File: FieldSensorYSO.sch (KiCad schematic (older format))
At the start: 3 parts, among them J1 22-28-4023, J2 22-28-4023, Y1 Field_Sensor_54_22

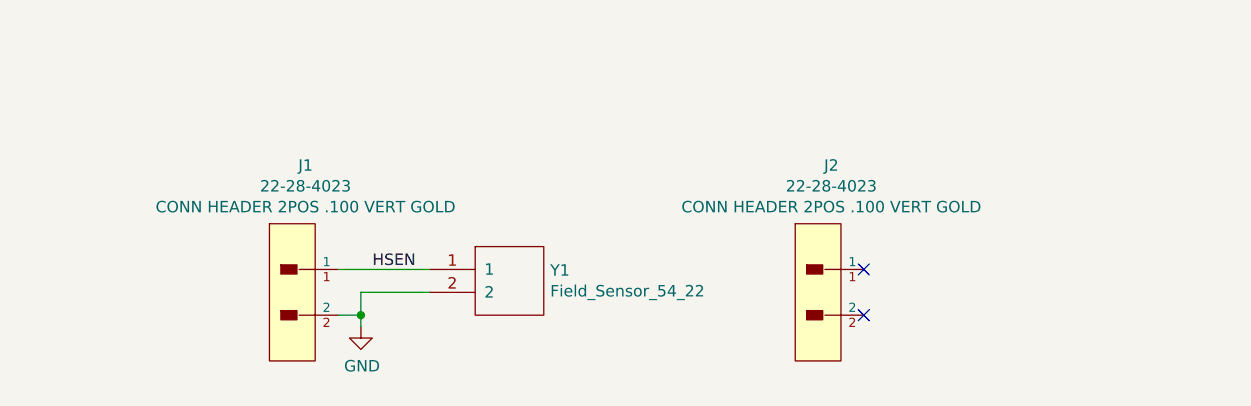
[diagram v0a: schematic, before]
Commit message: rev 2
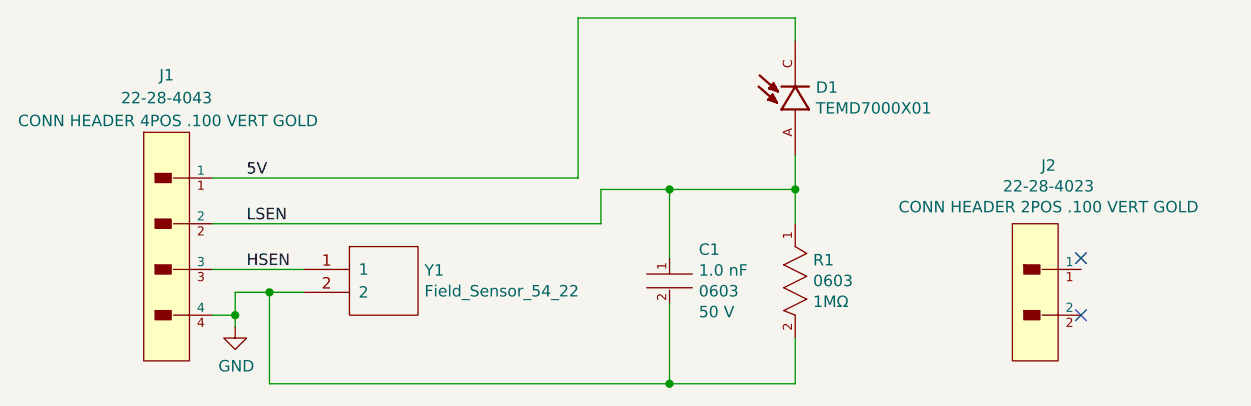
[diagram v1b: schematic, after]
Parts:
- removed J1: 22-28-4023, project:Molex-22-28-4023-0-0-0, symbol project:22-28-4023
- added C1: CC0603KRX7R9BB102, project:YAGEO-CC0603-0-0-0, symbol project:CC0603KRX7R9BB102
- added D1: TEMD7000X01, project:XDCR_TEMD7000X01, symbol project:TEMD7000X01
- added J1: 22-28-4043, project:Molex-SD-42375-001-0-0-0, symbol project:22-28-4043
- added R1: RC0603FR-071ML, project:Yageo-RC0603-0-0-IPC_A, symbol project:RC0603FR-071ML
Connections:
- net GND: now also C1.2, J1.4, R1.2
- net HSEN: now also J1.3
- new net 5V: D1.C, J1.1
- new net LSEN: C1.1, D1.A, J1.2, R1.1
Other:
- moved on the sheet: J2, Y1
